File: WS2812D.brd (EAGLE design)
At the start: 16.5 x 34.3 mm, 5 parts

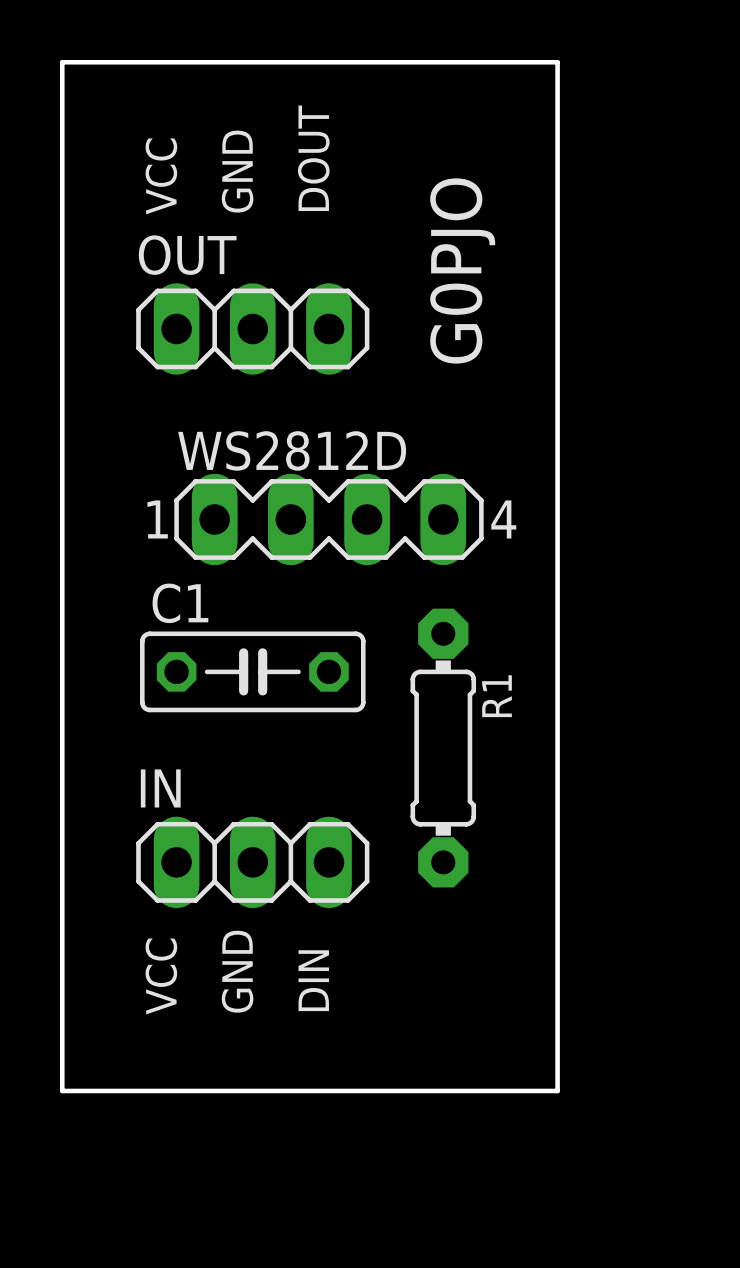
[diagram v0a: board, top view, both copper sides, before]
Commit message: More changes
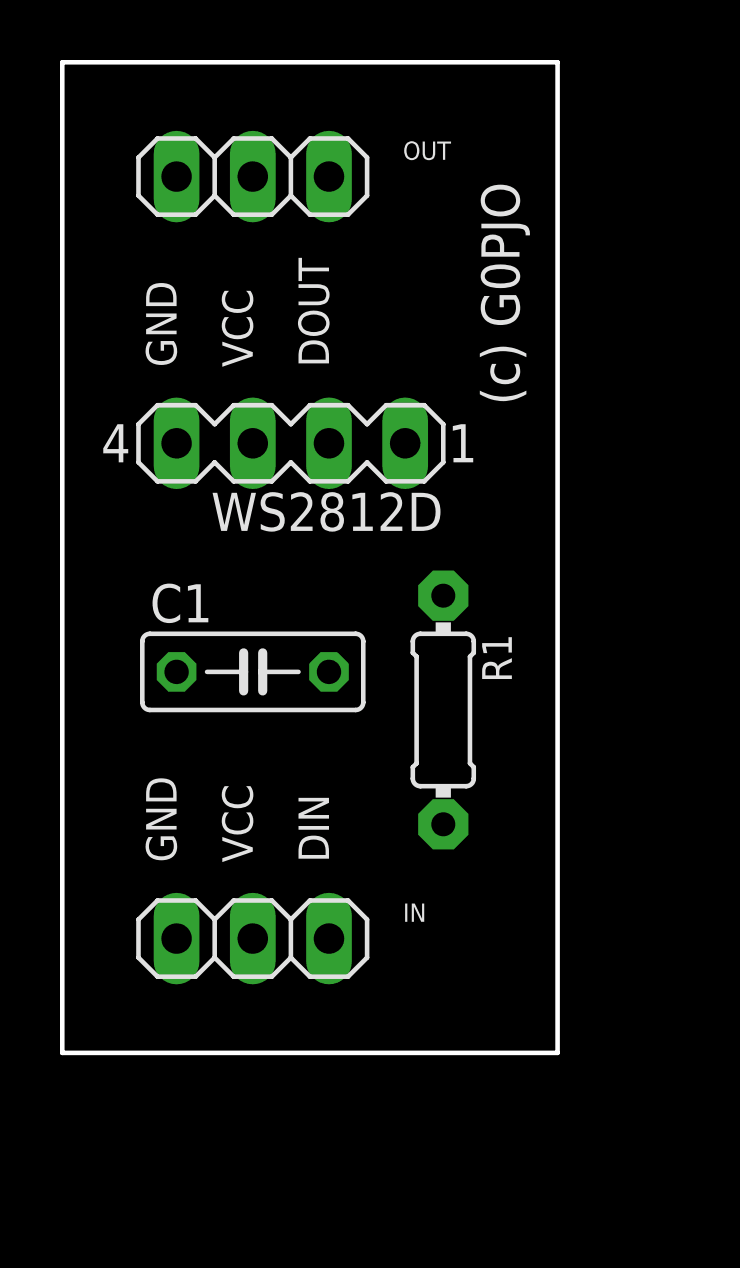
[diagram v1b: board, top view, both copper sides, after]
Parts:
- moved OUT 5.08 mm to (11.4, 67.3)
- moved WS2812D 2.84 mm to (12.7, 58.4), turned to 180 degrees
- moved IN 2.54 mm to (11.4, 41.9)
- moved R1 1.27 mm to (17.8, 49.5)
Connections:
- net S$1: now also IN.1, OUT.1, WS2812D.3; no longer IN.2, OUT.2, WS2812D.2
- net S$2: now also IN.2, OUT.2, WS2812D.2; no longer IN.1, OUT.1, WS2812D.3
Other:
- board size 16.5 x 34.3 mm -> 16.5 x 33 mm
- board text added: "(c) G0PJO"
- board text removed: "G0PJO"
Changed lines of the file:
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@@
 <board>
 <plain>
-<text x="8.89" y="39.37" size="1.016" layer="25" rot="R90">VCC</text>
-<text x="8.89" y="66.04" size="1.016" layer="25" rot="R90">VCC</text>
-<text x="11.43" y="66.04" size="1.016" layer="25" rot="R90">GND</text>
-<text x="11.43" y="39.37" size="1.016" layer="25" rot="R90">GND</text>
-<text x="13.97" y="39.37" size="1.016" layer="25" rot="R90">DIN</text>
-<text x="13.97" y="66.04" size="1.016" layer="25" rot="R90">DOUT</text>
+<text x="11.43" y="44.45" size="1.016" layer="25" rot="R90">VCC</text>
+<text x="11.43" y="60.96" size="1.016" layer="25" rot="R90">VCC</text>
+<text x="8.89" y="60.96" size="1.016" layer="25" rot="R90">GND</text>
+<text x="8.89" y="44.45" size="1.016" layer="25" rot="R90">GND</text>
+<text x="13.97" y="44.45" size="1.016" layer="25" rot="R90">DIN</text>
+<text x="13.97" y="60.96" size="1.016" layer="25" rot="R90">DOUT</text>
 <wire x1="5.08" y1="71.12" x2="21.59" y2="71.12" width="0.1524" layer="20"/>
-<wire x1="21.59" y1="71.12" x2="21.59" y2="36.83" width="0.1524" layer="20"/>
-<wire x1="21.59" y1="36.83" x2="5.08" y2="36.83" width="0.1524" layer="20"/>
-<wire x1="5.08" y1="36.83" x2="5.08" y2="71.12" width="0.1524" layer="20"/>
-<text x="19.05" y="60.96" size="1.6764" layer="25" rot="R90">G0PJO</text>
+<wire x1="21.59" y1="71.12" x2="21.59" y2="38.1" width="0.1524" layer="20"/>
+<wire x1="21.59" y1="38.1" x2="5.08" y2="38.1" width="0.1524" layer="20"/>
+<wire x1="5.08" y1="38.1" x2="5.08" y2="71.12" width="0.1524" layer="20"/>
+<text x="20.32" y="59.69" size="1.27" layer="25" rot="R90">(c) G0PJO</text>
 </plain>
 <attributes>
@@
 </autorouter>
 <elements>
-<element name="WS2812D" library="con-lstb" library_urn="urn:adsk.eagle:library:162" package="MA04-1" package3d_urn="urn:adsk.eagle:package:8337/1" value="" x="13.97" y="55.88" smashed="yes">
-<attribute name="NAME" x="8.89" y="57.531" size="1.27" layer="25" ratio="10"/>
-<attribute name="VALUE" x="14.605" y="57.531" size="1.27" layer="27" ratio="10"/>
-</element>
-<element name="R1" library="Clean-Kong" package="0204/7" value="75" x="17.78" y="48.26" smashed="yes" rot="R270">
-<attribute name="NAME" x="19.0754" y="50.8" size="0.9906" layer="25" ratio="10" rot="R270"/>
-<attribute name="VALUE" x="17.2974" y="49.8856" size="0.9906" layer="27" ratio="10" rot="R270"/>
+<element name="WS2812D" library="con-lstb" library_urn="urn:adsk.eagle:library:162" package="MA04-1" package3d_urn="urn:adsk.eagle:package:8337/1" value="" x="12.7" y="58.42" smashed="yes" rot="R180">
+<attribute name="NAME" x="17.78" y="56.769" size="1.27" layer="25" ratio="10" rot="R180"/>
+<attribute name="VALUE" x="12.065" y="56.769" size="1.27" layer="27" ratio="10" rot="R180"/>
+</element>
+<element name="R1" library="Clean-Kong" package="0204/7" value="75" x="17.78" y="49.53" smashed="yes" rot="R270">
+<attribute name="NAME" x="19.0754" y="52.07" size="0.9906" layer="25" ratio="10" rot="R270"/>
+<attribute name="VALUE" x="17.2974" y="51.1556" size="0.9906" layer="27" ratio="10" rot="R270"/>
 </element>
 <element name="C1" library="Clean-Kong" package="C050-025X075" value="100nf" x="11.43" y="50.8" smashed="yes">
@@
 <attribute name="VALUE" x="8.001" y="48.006" size="1.27" layer="27" ratio="10"/>
 </element>
-<element name="OUT" library="pinhead" library_urn="urn:adsk.eagle:library:325" package="1X03" package3d_urn="urn:adsk.eagle:package:22458/2" value="" x="11.43" y="62.23" smashed="yes">
-<attribute name="NAME" x="7.5438" y="64.0588" size="1.27" layer="25" ratio="10"/>
-<attribute name="VALUE" x="7.62" y="59.055" size="1.27" layer="27"/>
-</element>
-<element name="IN" library="pinhead" library_urn="urn:adsk.eagle:library:325" package="1X03" package3d_urn="urn:adsk.eagle:package:22458/2" value="" x="11.43" y="44.45" smashed="yes">
-<attribute name="NAME" x="7.5438" y="46.2788" size="1.27" layer="25" ratio="10"/>
-<attribute name="VALUE" x="7.62" y="41.275" size="1.27" layer="27"/>
+<element name="OUT" library="pinhead" library_urn="urn:adsk.eagle:library:325" package="1X03" package3d_urn="urn:adsk.eagle:package:22458/2" value="" x="11.43" y="67.31" smashed="yes">
+<attribute name="NAME" x="16.4338" y="67.8688" size="0.6096" layer="25" ratio="10"/>
+<attribute name="VALUE" x="7.62" y="64.135" size="1.27" layer="27"/>
+</element>
+<element name="IN" library="pinhead" library_urn="urn:adsk.eagle:library:325" package="1X03" package3d_urn="urn:adsk.eagle:package:22458/2" value="" x="11.43" y="41.91" smashed="yes">
+<attribute name="NAME" x="16.4338" y="42.4688" size="0.6096" layer="25" ratio="10"/>
+<attribute name="VALUE" x="7.62" y="38.735" size="1.27" layer="27"/>
 </element>
 </elements>
 <signals>
-<signal name="S$1">
-<contactref element="WS2812D" pad="2"/>
-<contactref element="C1" pad="1"/>
-<contactref element="OUT" pad="2"/>
-<contactref element="IN" pad="2"/>
-<wire x1="12.7" y1="55.88" x2="11.43" y2="62.23" width="0" layer="19" extent="1-1"/>
-<wire x1="8.89" y1="50.8" x2="12.7" y2="55.88" width="0" layer="19" extent="1-1"/>
-<wire x1="11.43" y1="44.45" x2="8.89" y2="50.8" width="0" layer="19" extent="1-1"/>
-</signal>
-<signal name="S$2">
-<contactref element="C1" pad="2"/>
-<contactref element="WS2812D" pad="3"/>
-<contactref element="OUT" pad="1"/>
-<contactref element="IN" pad="1"/>
-<wire x1="15.24" y1="55.88" x2="8.89" y2="62.23" width="0" layer="19" extent="1-1"/>
-<wire x1="13.97" y1="50.8" x2="15.24" y2="55.88" width="0" layer="19" extent="1-1"/>
-<wire x1="8.89" y1="44.45" x2="13.97" y2="50.8" width="0" layer="19" extent="1-1"/>
-</signal>
-<signal name="S$3">
-<contactref element="OUT" pad="3"/>
-<contactref element="WS2812D" pad="1"/>
-<wire x1="10.16" y1="55.88" x2="13.97" y2="62.23" width="0" layer="19" extent="1-1"/>
-</signal>
 <signal name="S$4">
 <contactref element="R1" pad="2"/>
 <contactref element="IN" pad="3"/>
-<wire x1="13.97" y1="44.45" x2="17.78" y2="44.45" width="0" layer="19" extent="1-1"/>
+<wire x1="13.97" y1="41.91" x2="17.78" y2="45.72" width="0" layer="19" extent="1-1"/>
 </signal>
 <signal name="S$5">
 <contactref element="WS2812D" pad="4"/>
 <contactref element="R1" pad="1"/>
-<wire x1="17.78" y1="55.88" x2="17.78" y2="52.07" width="0" layer="19" extent="1-1"/>
+<wire x1="8.89" y1="58.42" x2="17.78" y2="53.34" width="0" layer="19" extent="1-1"/>
+</signal>
+<signal name="S$1">
+<contactref element="C1" pad="1"/>
+<contactref element="IN" pad="1"/>
+<contactref element="WS2812D" pad="3"/>
+<contactref element="OUT" pad="1"/>
+<wire x1="11.43" y1="58.42" x2="8.89" y2="67.31" width="0" layer="19" extent="1-1"/>
+<wire x1="8.89" y1="50.8" x2="11.43" y2="58.42" width="0" layer="19" extent="1-1"/>
+<wire x1="8.89" y1="41.91" x2="8.89" y2="50.8" width="0" layer="19" extent="1-1"/>
+</signal>
+<signal name="S$2">
+<contactref element="WS2812D" pad="2"/>
+<contactref element="OUT" pad="2"/>
+<contactref element="C1" pad="2"/>
+<contactref element="IN" pad="2"/>
+<wire x1="13.97" y1="58.42" x2="11.43" y2="67.31" width="0" layer="19" extent="1-1"/>
+<wire x1="13.97" y1="50.8" x2="13.97" y2="58.42" width="0" layer="19" extent="1-1"/>
+<wire x1="11.43" y1="41.91" x2="13.97" y2="50.8" width="0" layer="19" extent="1-1"/>
+</signal>
+<signal name="S$3">
+<contactref element="WS2812D" pad="1"/>
+<contactref element="OUT" pad="3"/>
+<wire x1="16.51" y1="58.42" x2="13.97" y2="67.31" width="0" layer="19" extent="1-1"/>
 </signal>
 </signals>

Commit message: More PCB
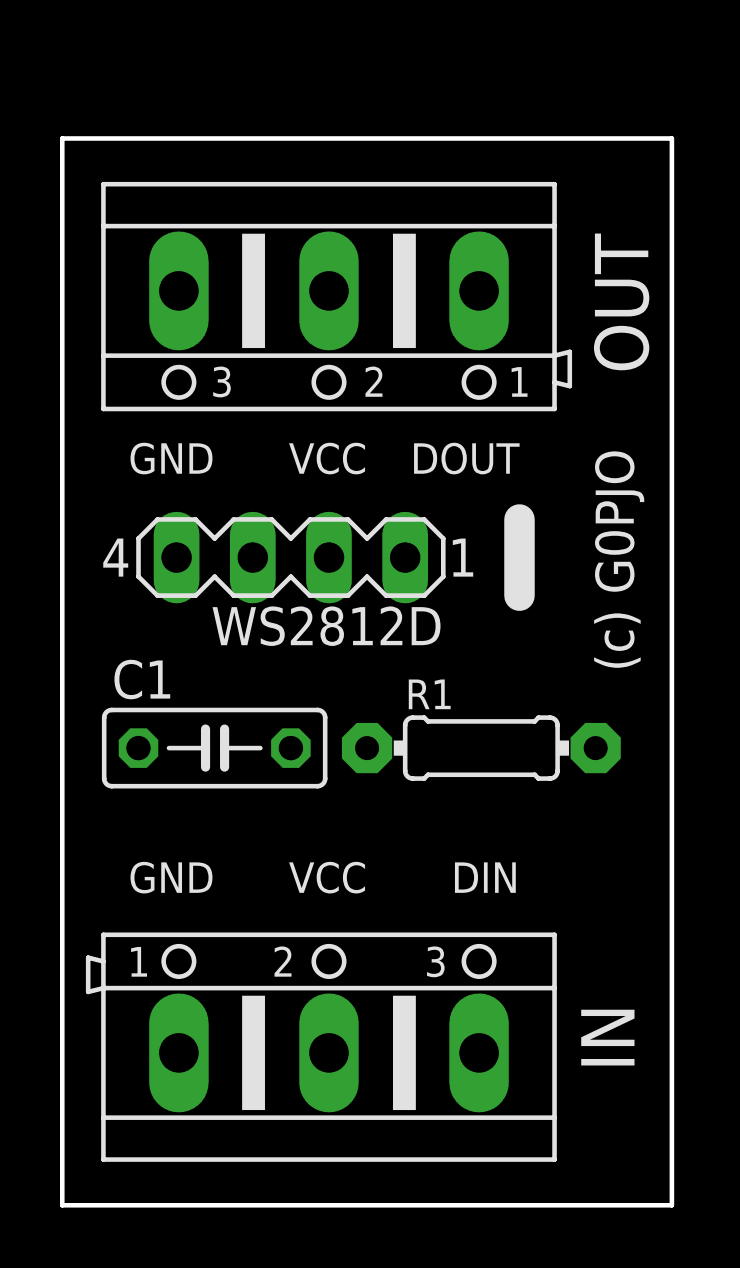
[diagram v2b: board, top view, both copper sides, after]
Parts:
- IN, OUT: device pinhead:1X03 -> con-ptr500:AK500/3
- moved OUT 4.58 mm to (14.0, 63.5), turned to 180 degrees
- moved IN 4.58 mm to (14.0, 38.1)
- moved WS2812D 3.81 mm to (12.7, 54.6)
- moved C1 2.84 mm to (10.2, 48.3)
- moved R1 1.80 mm to (19.1, 48.3), turned to 0 degrees
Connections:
- net S$1: now also OUT.3; no longer OUT.1
- net S$3: now also OUT.1; no longer OUT.3
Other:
- board size 16.5 x 33 mm -> 20.3 x 35.6 mm
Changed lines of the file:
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@@
 <board>
 <plain>
-<text x="11.43" y="44.45" size="1.016" layer="25" rot="R90">VCC</text>
-<text x="11.43" y="60.96" size="1.016" layer="25" rot="R90">VCC</text>
-<text x="8.89" y="60.96" size="1.016" layer="25" rot="R90">GND</text>
-<text x="8.89" y="44.45" size="1.016" layer="25" rot="R90">GND</text>
-<text x="13.97" y="44.45" size="1.016" layer="25" rot="R90">DIN</text>
-<text x="13.97" y="60.96" size="1.016" layer="25" rot="R90">DOUT</text>
-<wire x1="5.08" y1="71.12" x2="21.59" y2="71.12" width="0.1524" layer="20"/>
-<wire x1="21.59" y1="71.12" x2="21.59" y2="38.1" width="0.1524" layer="20"/>
-<wire x1="21.59" y1="38.1" x2="5.08" y2="38.1" width="0.1524" layer="20"/>
-<wire x1="5.08" y1="38.1" x2="5.08" y2="71.12" width="0.1524" layer="20"/>
-<text x="20.32" y="59.69" size="1.27" layer="25" rot="R90">(c) G0PJO</text>
+<text x="15.24" y="44.45" size="1.016" layer="25" rot="R180">VCC</text>
+<text x="15.24" y="58.42" size="1.016" layer="25" rot="R180">VCC</text>
+<text x="10.16" y="58.42" size="1.016" layer="25" rot="R180">GND</text>
+<text x="10.16" y="44.45" size="1.016" layer="25" rot="R180">GND</text>
+<text x="20.32" y="44.45" size="1.016" layer="25" rot="R180">DIN</text>
+<text x="20.32" y="58.42" size="1.016" layer="25" rot="R180">DOUT</text>
+<wire x1="5.08" y1="68.58" x2="25.4" y2="68.58" width="0.1524" layer="20"/>
+<wire x1="25.4" y1="68.58" x2="25.4" y2="33.02" width="0.1524" layer="20"/>
+<wire x1="25.4" y1="33.02" x2="5.08" y2="33.02" width="0.1524" layer="20"/>
+<wire x1="5.08" y1="33.02" x2="5.08" y2="68.58" width="0.1524" layer="20"/>
+<text x="24.13" y="50.8" size="1.27" layer="25" rot="R90">(c) G0PJO</text>
+<wire x1="20.32" y1="55.88" x2="20.32" y2="53.34" width="1.016" layer="25"/>
 </plain>
 <attributes>
@@
 </autorouter>
 <elements>
-<element name="WS2812D" library="con-lstb" library_urn="urn:adsk.eagle:library:162" package="MA04-1" package3d_urn="urn:adsk.eagle:package:8337/1" value="" x="12.7" y="58.42" smashed="yes" rot="R180">
-<attribute name="NAME" x="17.78" y="56.769" size="1.27" layer="25" ratio="10" rot="R180"/>
-<attribute name="VALUE" x="12.065" y="56.769" size="1.27" layer="27" ratio="10" rot="R180"/>
-</element>
-<element name="R1" library="Clean-Kong" package="0204/7" value="75" x="17.78" y="49.53" smashed="yes" rot="R270">
-<attribute name="NAME" x="19.0754" y="52.07" size="0.9906" layer="25" ratio="10" rot="R270"/>
-<attribute name="VALUE" x="17.2974" y="51.1556" size="0.9906" layer="27" ratio="10" rot="R270"/>
-</element>
-<element name="C1" library="Clean-Kong" package="C050-025X075" value="100nf" x="11.43" y="50.8" smashed="yes">
-<attribute name="NAME" x="8.001" y="52.451" size="1.27" layer="25" ratio="10"/>
-<attribute name="VALUE" x="8.001" y="48.006" size="1.27" layer="27" ratio="10"/>
-</element>
-<element name="OUT" library="pinhead" library_urn="urn:adsk.eagle:library:325" package="1X03" package3d_urn="urn:adsk.eagle:package:22458/2" value="" x="11.43" y="67.31" smashed="yes">
-<attribute name="NAME" x="16.4338" y="67.8688" size="0.6096" layer="25" ratio="10"/>
-<attribute name="VALUE" x="7.62" y="64.135" size="1.27" layer="27"/>
-</element>
-<element name="IN" library="pinhead" library_urn="urn:adsk.eagle:library:325" package="1X03" package3d_urn="urn:adsk.eagle:package:22458/2" value="" x="11.43" y="41.91" smashed="yes">
-<attribute name="NAME" x="16.4338" y="42.4688" size="0.6096" layer="25" ratio="10"/>
-<attribute name="VALUE" x="7.62" y="38.735" size="1.27" layer="27"/>
+<element name="WS2812D" library="con-lstb" library_urn="urn:adsk.eagle:library:162" package="MA04-1" package3d_urn="urn:adsk.eagle:package:8337/1" value="" x="12.7" y="54.61" smashed="yes" rot="R180">
+<attribute name="NAME" x="17.78" y="52.959" size="1.27" layer="25" ratio="10" rot="R180"/>
+<attribute name="VALUE" x="12.065" y="52.959" size="1.27" layer="27" ratio="10" rot="R180"/>
+</element>
+<element name="R1" library="Clean-Kong" package="0204/7" value="75" x="19.05" y="48.26" smashed="yes">
+<attribute name="NAME" x="16.51" y="49.5554" size="0.9906" layer="25" ratio="10"/>
+<attribute name="VALUE" x="17.4244" y="47.7774" size="0.9906" layer="27" ratio="10"/>
+</element>
+<element name="C1" library="Clean-Kong" package="C050-025X075" value="100nf" x="10.16" y="48.26" smashed="yes">
+<attribute name="NAME" x="6.731" y="49.911" size="1.27" layer="25" ratio="10"/>
+<attribute name="VALUE" x="6.731" y="45.466" size="1.27" layer="27" ratio="10"/>
+</element>
+<element name="IN" library="con-ptr500" library_urn="urn:adsk.eagle:library:181" package="AK500/3" package3d_urn="urn:adsk.eagle:package:9883/1" value="" x="13.97" y="38.1" smashed="yes">
+<attribute name="NAME" x="24.1554" y="37.465" size="1.778" layer="25" ratio="10" rot="R90"/>
+<attribute name="VALUE" x="6.3754" y="32.385" size="1.778" layer="27" ratio="10"/>
+</element>
+<element name="OUT" library="con-ptr500" library_urn="urn:adsk.eagle:library:181" package="AK500/3" package3d_urn="urn:adsk.eagle:package:9883/1" value="" x="13.97" y="63.5" smashed="yes" rot="R180">
+<attribute name="NAME" x="22.8346" y="65.405" size="1.778" layer="25" ratio="10" rot="R270"/>
+<attribute name="VALUE" x="21.5646" y="69.215" size="1.778" layer="27" ratio="10" rot="R180"/>
 </element>
 </elements>
@@
 <contactref element="R1" pad="2"/>
 <contactref element="IN" pad="3"/>
-<wire x1="13.97" y1="41.91" x2="17.78" y2="45.72" width="0" layer="19" extent="1-1"/>
+<wire x1="18.9738" y1="38.1" x2="22.86" y2="48.26" width="0" layer="19" extent="1-1"/>
 </signal>
 <signal name="S$5">
 <contactref element="WS2812D" pad="4"/>
 <contactref element="R1" pad="1"/>
-<wire x1="8.89" y1="58.42" x2="17.78" y2="53.34" width="0" layer="19" extent="1-1"/>
+<wire x1="15.24" y1="48.26" x2="8.89" y2="54.61" width="0" layer="19" extent="1-1"/>
 </signal>
 <signal name="S$1">
 <contactref element="C1" pad="1"/>
+<contactref element="WS2812D" pad="3"/>
+<contactref element="OUT" pad="3"/>
 <contactref element="IN" pad="1"/>
-<contactref element="WS2812D" pad="3"/>
-<contactref element="OUT" pad="1"/>
-<wire x1="11.43" y1="58.42" x2="8.89" y2="67.31" width="0" layer="19" extent="1-1"/>
-<wire x1="8.89" y1="50.8" x2="11.43" y2="58.42" width="0" layer="19" extent="1-1"/>
-<wire x1="8.89" y1="41.91" x2="8.89" y2="50.8" width="0" layer="19" extent="1-1"/>
+<wire x1="11.43" y1="54.61" x2="8.9662" y2="63.5" width="0" layer="19" extent="1-1"/>
+<wire x1="7.62" y1="48.26" x2="11.43" y2="54.61" width="0" layer="19" extent="1-1"/>
+<wire x1="8.9662" y1="38.1" x2="7.62" y2="48.26" width="0" layer="19" extent="1-1"/>
 </signal>
 <signal name="S$2">
 <contactref element="WS2812D" pad="2"/>
+<contactref element="C1" pad="2"/>
 <contactref element="OUT" pad="2"/>
-<contactref element="C1" pad="2"/>
 <contactref element="IN" pad="2"/>
-<wire x1="13.97" y1="58.42" x2="11.43" y2="67.31" width="0" layer="19" extent="1-1"/>
-<wire x1="13.97" y1="50.8" x2="13.97" y2="58.42" width="0" layer="19" extent="1-1"/>
-<wire x1="11.43" y1="41.91" x2="13.97" y2="50.8" width="0" layer="19" extent="1-1"/>
+<wire x1="13.97" y1="54.61" x2="13.97" y2="63.5" width="0" layer="19" extent="1-1"/>
+<wire x1="12.7" y1="48.26" x2="13.97" y2="54.61" width="0" layer="19" extent="1-1"/>
+<wire x1="13.97" y1="38.1" x2="12.7" y2="48.26" width="0" layer="19" extent="1-1"/>
 </signal>
 <signal name="S$3">
 <contactref element="WS2812D" pad="1"/>
-<contactref element="OUT" pad="3"/>
-<wire x1="16.51" y1="58.42" x2="13.97" y2="67.31" width="0" layer="19" extent="1-1"/>
+<contactref element="OUT" pad="1"/>
+<wire x1="16.51" y1="54.61" x2="18.9738" y2="63.5" width="0" layer="19" extent="1-1"/>
 </signal>
 </signals>
